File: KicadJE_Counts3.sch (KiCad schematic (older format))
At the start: 78 parts, among them J201 ClockOut, J202 ClockIn, J203 Out0, J204 Out1, J205 Out2, J206 Out3, J207 Out4, J208 Out5, J209 Out6, J210 Out7, J211 Out8, J212 Out9, J213 Reset, J214 Hold, P201 HEADER_2x5_Doepfer, SW201 Run, U201 LM555, U202 4017

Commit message: major components placed for counter
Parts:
- C203: value 100uF 16v -> 10uF 16v; symbol Device:CP -> Device:C
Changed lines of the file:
@@
 $EndComp
 $Comp
-L Device:CP C?
+L Device:C C?
 U 1 1 5C783FA4
 P 2150 1250
@@
 AR Path="/5C781441/5C783FA4" Ref="C203"  Part="1"
 F 0 "C203" H 2100 1450 50  0000 L CNN
-F 1 "100uF 16v" H 2000 1550 50  0000 L CNN
+F 1 "10uF 16v" H 2000 1550 50  0000 L CNN
 F 2 "Capacitor_SMD:C_1206_3216Metric" H 2188 1100 50  0001 C CNN
 F 3 "~" H 2150 1250 50  0001 C CNN

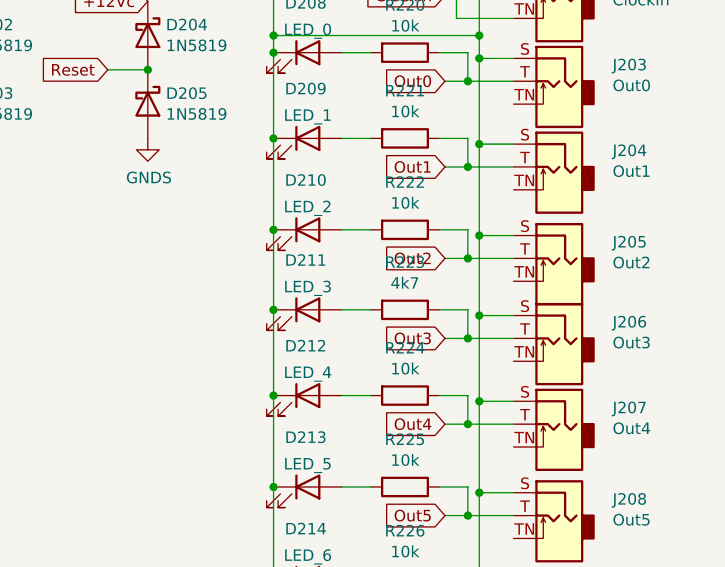
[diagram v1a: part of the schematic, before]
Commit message: Update KicadJE_Counts3.sch
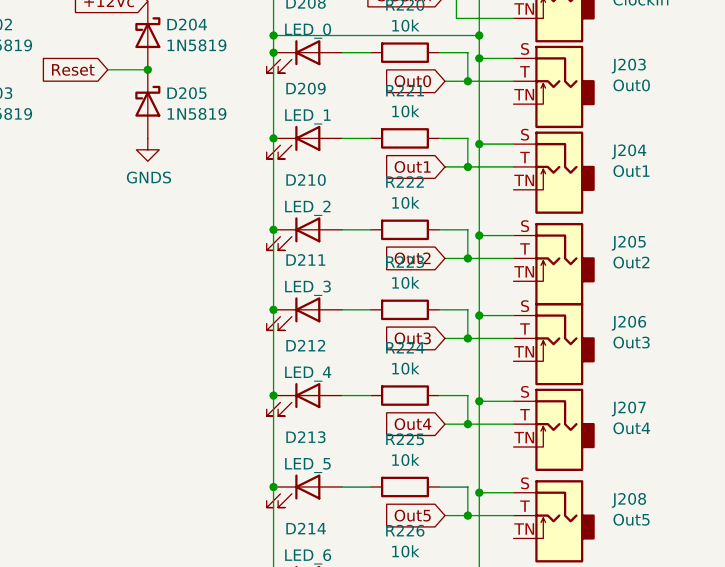
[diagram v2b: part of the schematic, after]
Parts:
- R223: value 4k7 -> 10k
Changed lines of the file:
@@
 AR Path="/5C781441/5C83D871" Ref="R223"  Part="1"
 F 0 "R223" V 9668 2800 50  0000 C CNN
-F 1 "4k7" V 9759 2800 50  0000 C CNN
+F 1 "10k" V 9759 2800 50  0000 C CNN
 F 2 "AJ:R_0805_AJ" V 9805 2800 50  0001 C CNN
 F 3 "~" H 9875 2800 50  0001 C CNN
